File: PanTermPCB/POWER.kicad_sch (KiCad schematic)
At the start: 5 parts, among them U2 SGM2212-3.3XKC3G/TR_C3294699

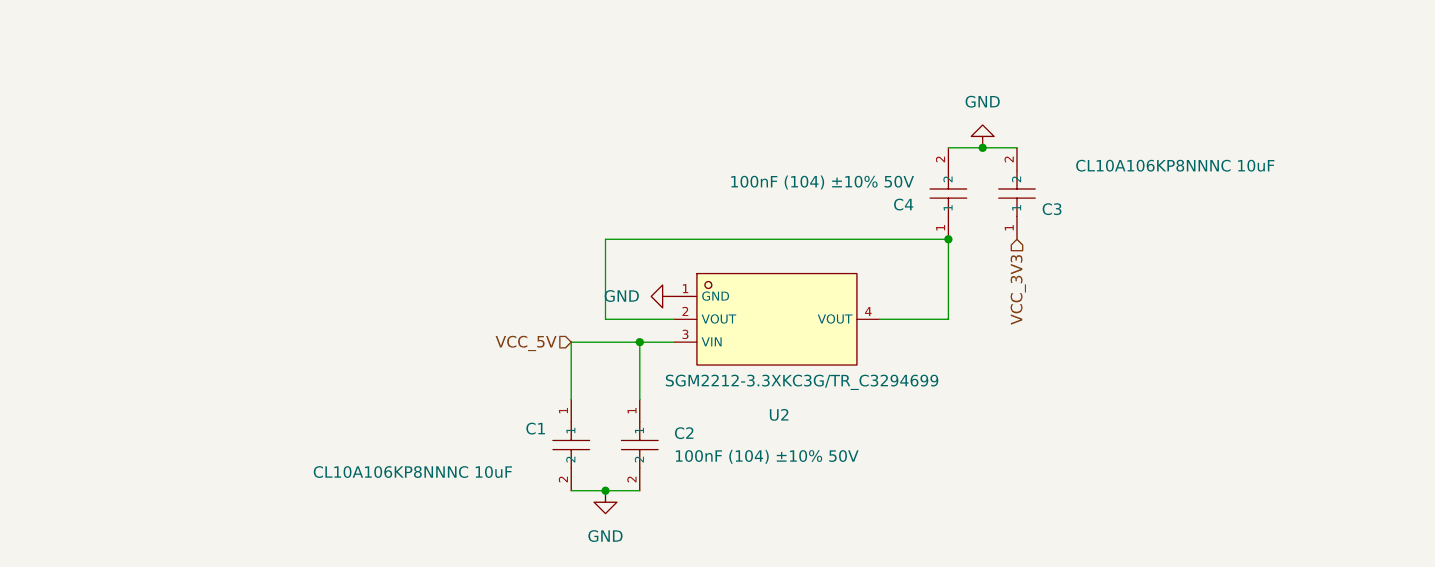
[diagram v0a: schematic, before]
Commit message: Battery charging IC
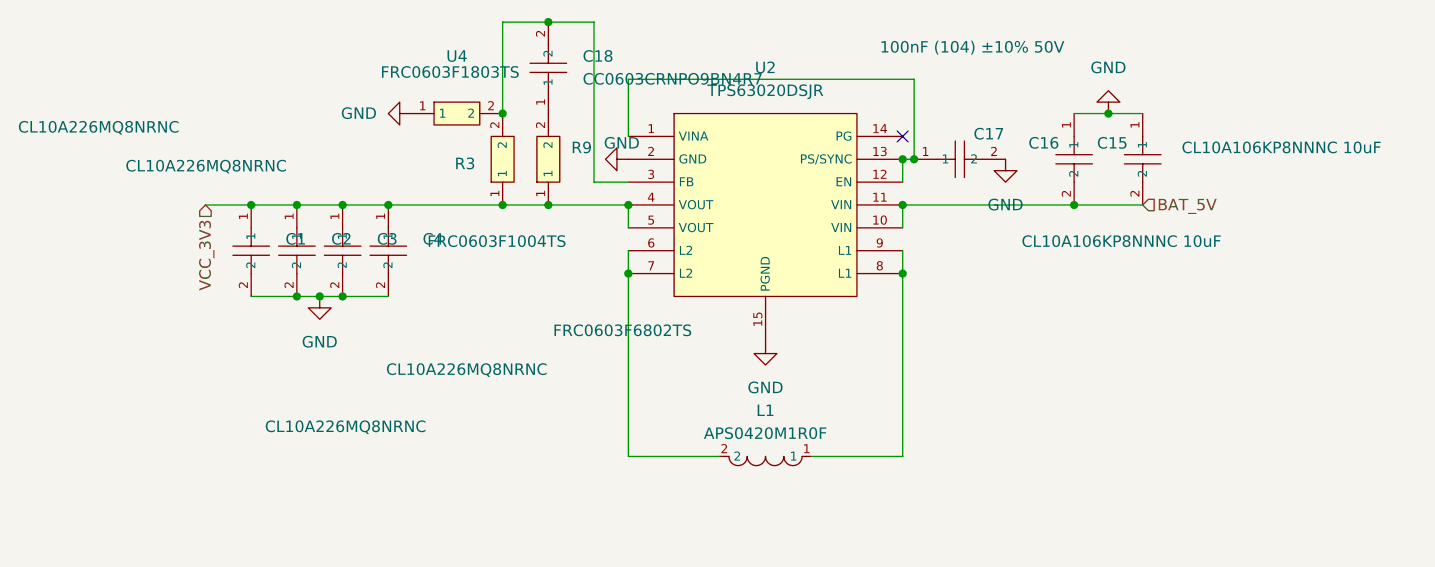
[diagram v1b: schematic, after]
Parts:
- removed C1, C3: CL10A106KP8NNNC 10uF, lcsc_footprints:C19702_C0603, symbol lcsc_imported:CL10A106KP8NNNC
- removed C2, C4: 100nF (104) ±10% 50V, lcsc_footprints:C1591_C0603, symbol lcsc_imported:100nF_(104)_±10%_50V
- removed U2: SGM2212-3.3XKC3G/TR_C3294699, lcsc_footprints:C3294699_SOT-223-3_L6_5-W3_4-P2_30-LS7_0-BR, symbol lcsc_imported:SGM2212-3_3XKC3G/TR_C3294699
- added C1, C2, C3, C4: CL10A226MQ8NRNC, lcsc_footprints:C59461_C0603, symbol lcsc_imported:CL10A226MQ8NRNC
- added C15, C16: CL10A106KP8NNNC 10uF, lcsc_footprints:C19702_C0603, symbol lcsc_imported:CL10A106KP8NNNC
- added C17: 100nF (104) ±10% 50V, lcsc_footprints:C1591_C0603, symbol lcsc_imported:100nF_(104)_±10%_50V
- added C18: CC0603CRNPO9BN4R7, lcsc_footprints:C282071_C0603, symbol lcsc_imported:CC0603CRNPO9BN4R7
- added L1: APS0420M1R0F, lcsc_footprints:C49261133_IND-SMD_L4_1-W4_1_PA5430, symbol lcsc_imported:APS0420M1R0F
- added R3: FRC0603F1004TS, lcsc_footprints:C2907003_R0603, symbol lcsc_imported:FRC0603F1004TS
- added R9: FRC0603F6802TS, lcsc_footprints:C2907063_R0603, symbol lcsc_imported:FRC0603F6802TS
- added U2: TPS63020DSJR, lcsc_footprints:C15483_VSON-14_L4_0-W3_0-P0_50-BL-EP_TI_DSJ, symbol lcsc_imported:TPS63020DSJR
- added U4: FRC0603F1803TS, lcsc_footprints:C2906999_R0603, symbol lcsc_imported:FRC0603F1803TS
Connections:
- net GND: now also C1.2, C15.1, C16.1, C17.2, C2.2, C3.2, C4.2, U2.15 (PGND), U2.2 (GND), U4.1
- net VCC_3V3: now also C1.1, C2.1, C3.1, C4.1, R3.1, R9.1, U2.4 (VOUT), U2.5 (VOUT)
- new net: C18.1, R9.2
- new net: C17.1, U2.1 (VINA), U2.12 (EN), U2.13 (PS/SYNC)
- new net: C18.2, R3.2, U2.3 (FB), U4.2
- new net: L1.2, U2.6 (L2), U2.7 (L2)
- new net: L1.1, U2.8 (L1), U2.9 (L1)
- new net BAT_5V: C15.2, C16.2, U2.10 (VIN), U2.11 (VIN)
- no-connect marks 0 -> 1
